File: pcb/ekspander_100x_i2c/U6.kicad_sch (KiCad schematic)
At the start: 5 parts, among them J15 DG127A-5.08-06P-14-00AH, J16 DG127A-5.08-06P-14-00AH, J17 DG127A-5.08-06P-14-00AH, U6 MCP23017_SP

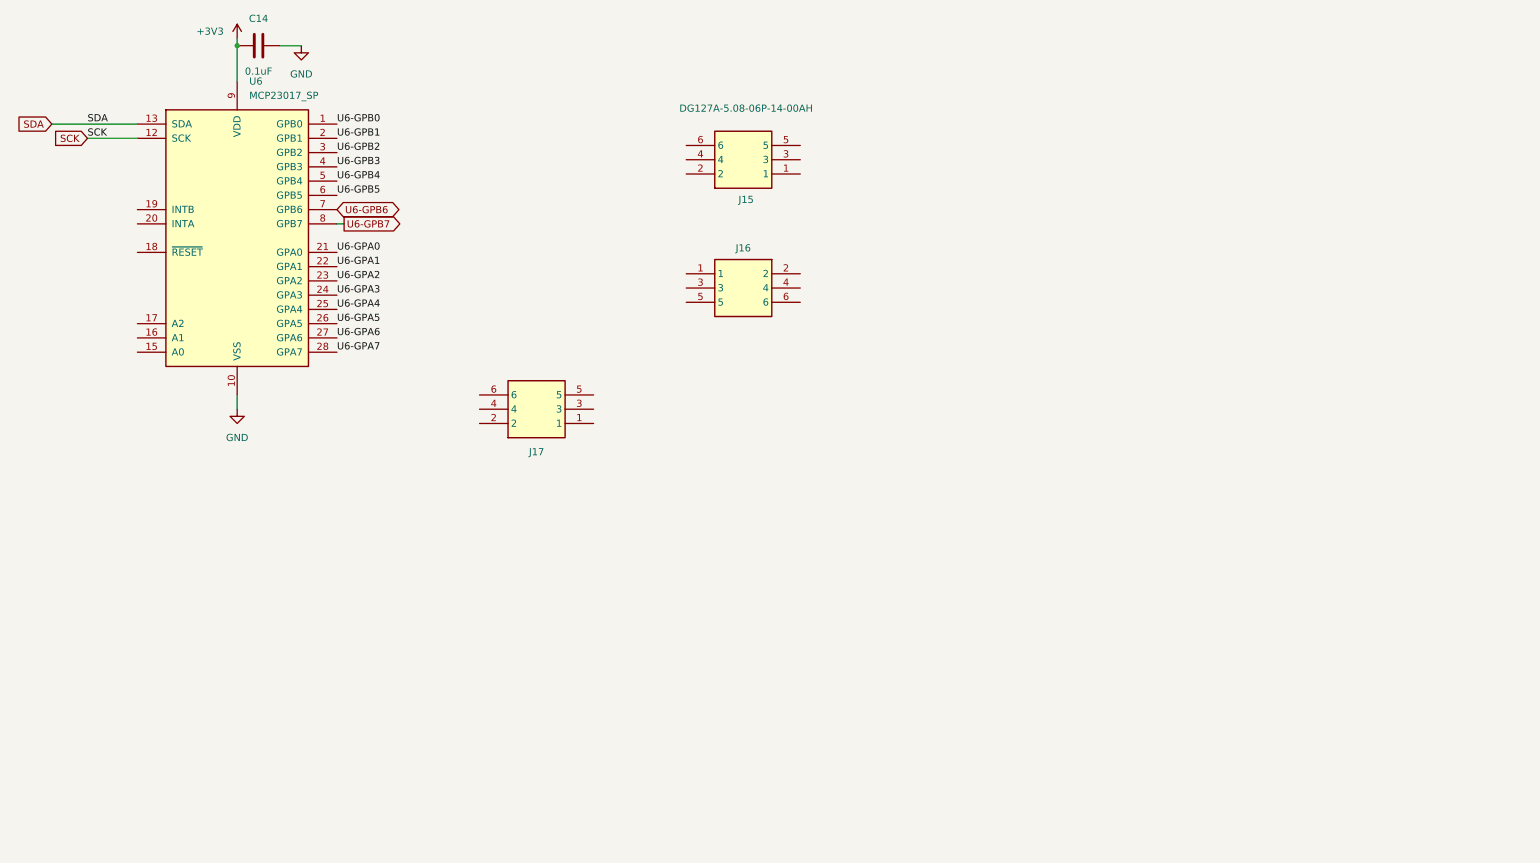
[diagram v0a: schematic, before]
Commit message: Ekspander U5 - U6 update
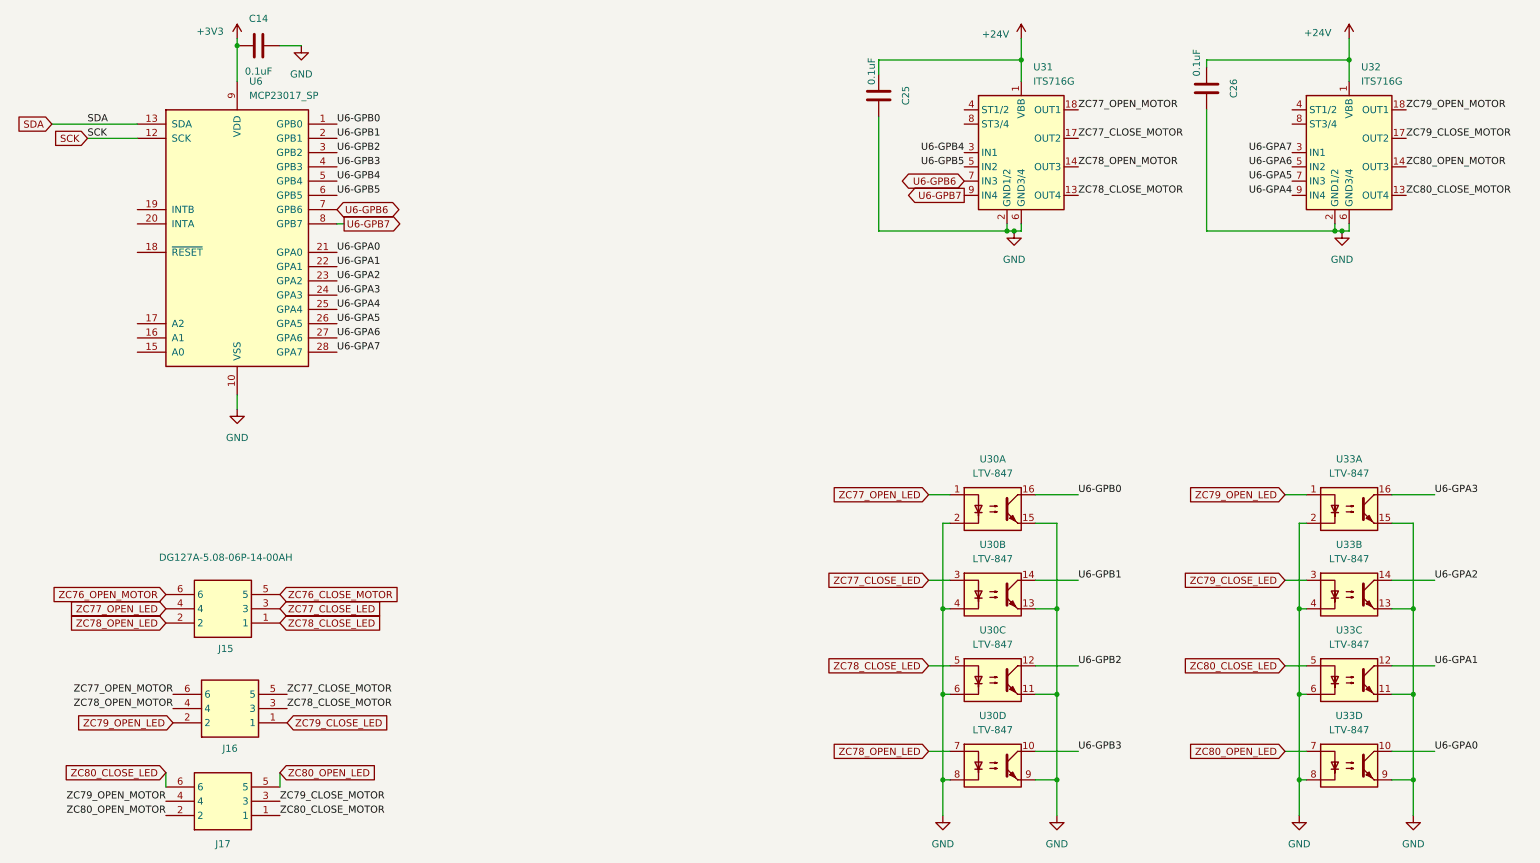
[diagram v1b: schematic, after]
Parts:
- added C25, C26: 0.1uF, Capacitor_SMD:C_0805_2012Metric_Pad1.18x1.45mm_HandSolder, symbol Device:C
- added U30, U33: LTV-847, Package_DIP:DIP-16_W7.62mm, symbol Isolator:LTV-847
- added U31, U32: ITS716G, Package_SO:SOIC-20W_7.5x12.8mm_P1.27mm, symbol Driver_FET:ITS716G
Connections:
- net GND: now also C25.2, C26.2, U30.11, U30.13, U30.15, U30.2, U30.4, U30.6, U30.8, U30.9, U31.2 (GND1/2), U31.6 (GND3/4), U32.2 (GND1/2), U32.6 (GND3/4), U33.11, U33.13, U33.15, U33.2, U33.4, U33.6, U33.8, U33.9
- net U6-GPA0: now also U33.10
- net U6-GPA1: now also U33.12
- net U6-GPA2: now also U33.14
- net U6-GPA3: now also U33.16
- net U6-GPA4: now also U32.9 (IN4)
- net U6-GPA5: now also U32.7 (IN3)
- net U6-GPA6: now also U32.5 (IN2)
- net U6-GPA7: now also U32.3 (IN1)
- net U6-GPB0: now also U30.16
- net U6-GPB1: now also U30.14
- net U6-GPB2: now also U30.12
- net U6-GPB3: now also U30.10
- net U6-GPB4: now also U31.3 (IN1)
- net U6-GPB5: now also U31.5 (IN2)
- net U6-GPB6: now also U31.7 (IN3)
- net U6-GPB7: now also U31.9 (IN4)
- net ZC79_CLOSE_LED: now reaches J16.1
- net ZC79_CLOSE_LED: now also U33.3
- net ZC79_OPEN_LED: now reaches J16.2
- net ZC79_OPEN_LED: now also U33.1
- net ZC78_CLOSE_MOTOR: now reaches J16.3
- net ZC78_CLOSE_MOTOR: now also U31.13 (OUT4)
- net ZC78_OPEN_MOTOR: now reaches J16.4
- net ZC78_OPEN_MOTOR: now also U31.14 (OUT3)
- net ZC77_CLOSE_MOTOR: now reaches J16.5
- net ZC77_CLOSE_MOTOR: now also U31.17 (OUT2)
- net ZC77_OPEN_MOTOR: now reaches J16.6
- net ZC77_OPEN_MOTOR: now also U31.18 (OUT1)
- net ZC78_CLOSE_LED: now reaches J15.1
- net ZC78_CLOSE_LED: now also U30.5
- net ZC78_OPEN_LED: now reaches J15.2
- net ZC78_OPEN_LED: now also U30.7
- net ZC77_CLOSE_LED: now reaches J15.3
- net ZC77_CLOSE_LED: now also U30.3
- net ZC77_OPEN_LED: now reaches J15.4
- net ZC77_OPEN_LED: now also U30.1
- net ZC76_CLOSE_MOTOR: now reaches J15.5
- net ZC76_OPEN_MOTOR: now reaches J15.6
- net ZC80_CLOSE_MOTOR: now reaches J17.1
- net ZC80_CLOSE_MOTOR: now also U32.13 (OUT4)
- net ZC80_OPEN_MOTOR: now reaches J17.2
- net ZC80_OPEN_MOTOR: now also U32.14 (OUT3)
- net ZC79_CLOSE_MOTOR: now reaches J17.3
- net ZC79_CLOSE_MOTOR: now also U32.17 (OUT2)
- net ZC79_OPEN_MOTOR: now reaches J17.4
- net ZC79_OPEN_MOTOR: now also U32.18 (OUT1)
- net ZC80_OPEN_LED: now reaches J17.5
- net ZC80_OPEN_LED: now also U33.7
- net ZC80_CLOSE_LED: now reaches J17.6
- net ZC80_CLOSE_LED: now also U33.5
- new net +24V: C25.1, C26.1, U31.1 (VBB), U31.10 (VBB), U31.11 (VBB), U31.12 (VBB), U31.15 (VBB), U31.16 (VBB), U31.19 (VBB), U31.20 (VBB), U32.1 (VBB), U32.10 (VBB), U32.11 (VBB), U32.12 (VBB), U32.15 (VBB), U32.16 (VBB), U32.19 (VBB), U32.20 (VBB)
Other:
- moved on the sheet: J15, J16, J17
